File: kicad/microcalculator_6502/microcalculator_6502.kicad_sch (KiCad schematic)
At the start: 51 parts, among them J1 /SO, J10 CA, J11 IRQ_EXT_0, J12 IRQ_EXT_1, J13 CB, J14 D[7...0], J15 AUXILIARE, J16 RX_C, J17 TX_D, J18 RX_D, J2 A[11...0], J3 A[15...12], J4 D[7...0], J5 /ML, J6 /VP, J7 SYNC, J8 D[7...0], J9 /NMI, SW1 RESET, U1 65C02, U2 65C22, U3 65C51, U4 62256, U5 28C256, U6 74LS08, U7 74LS73, U8 ATF22V10C-15PU, Y1 CXO_DIP14, Y2 CXO_DIP8

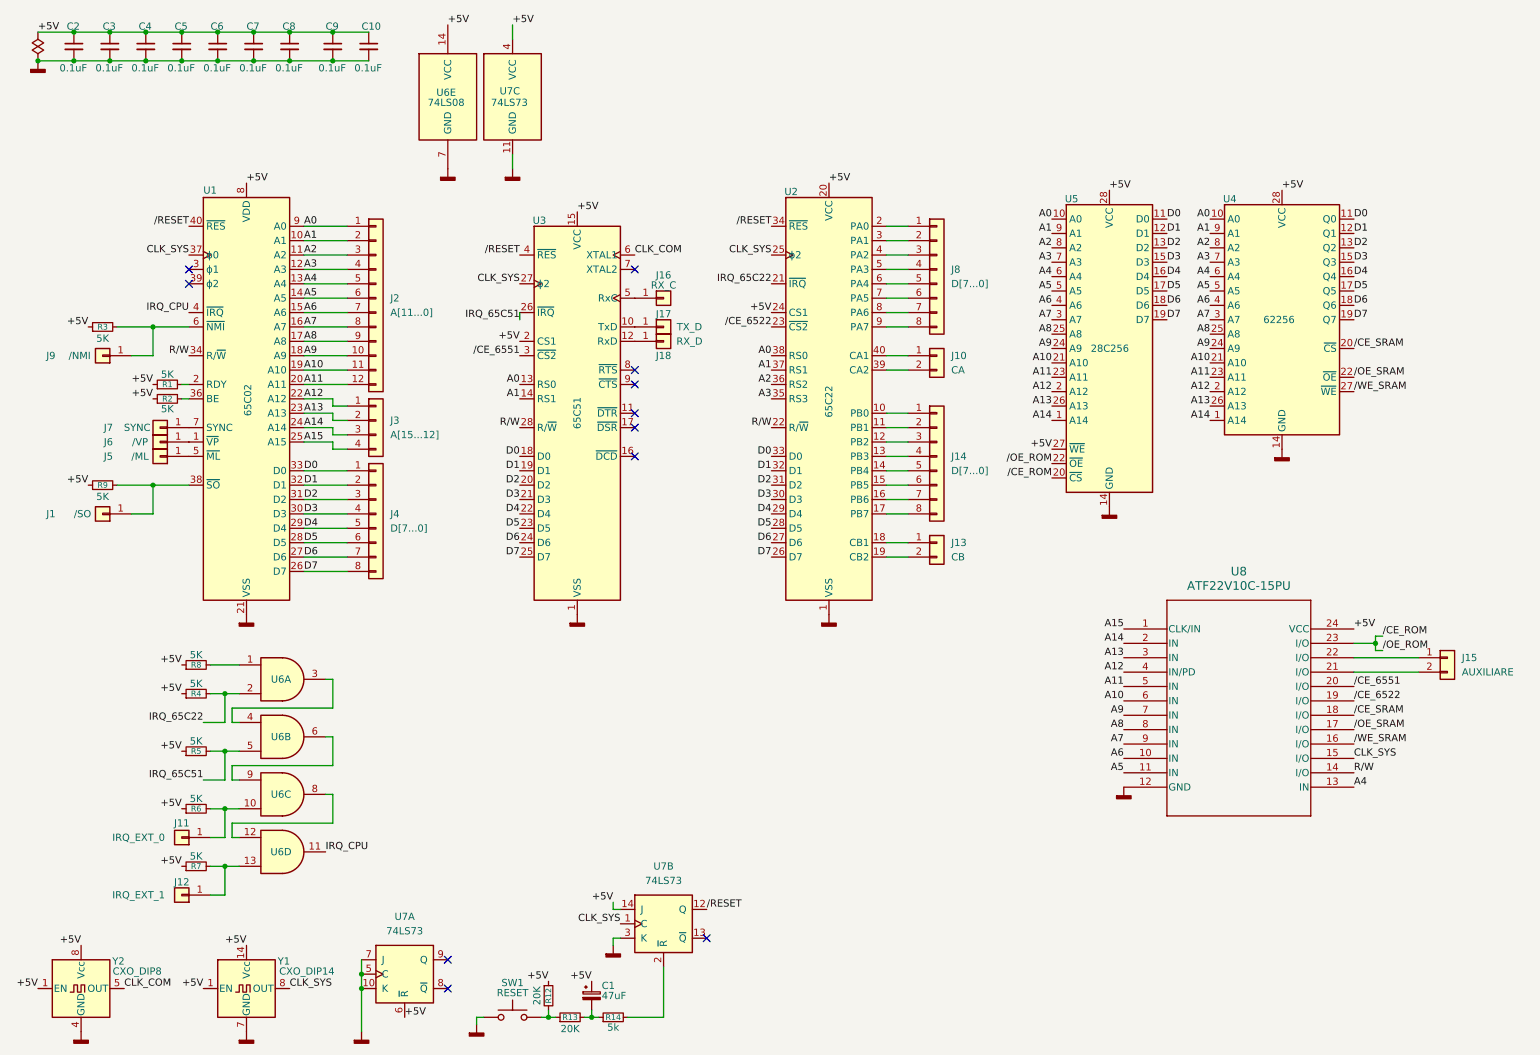
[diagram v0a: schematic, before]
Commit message: diagrama actualizata
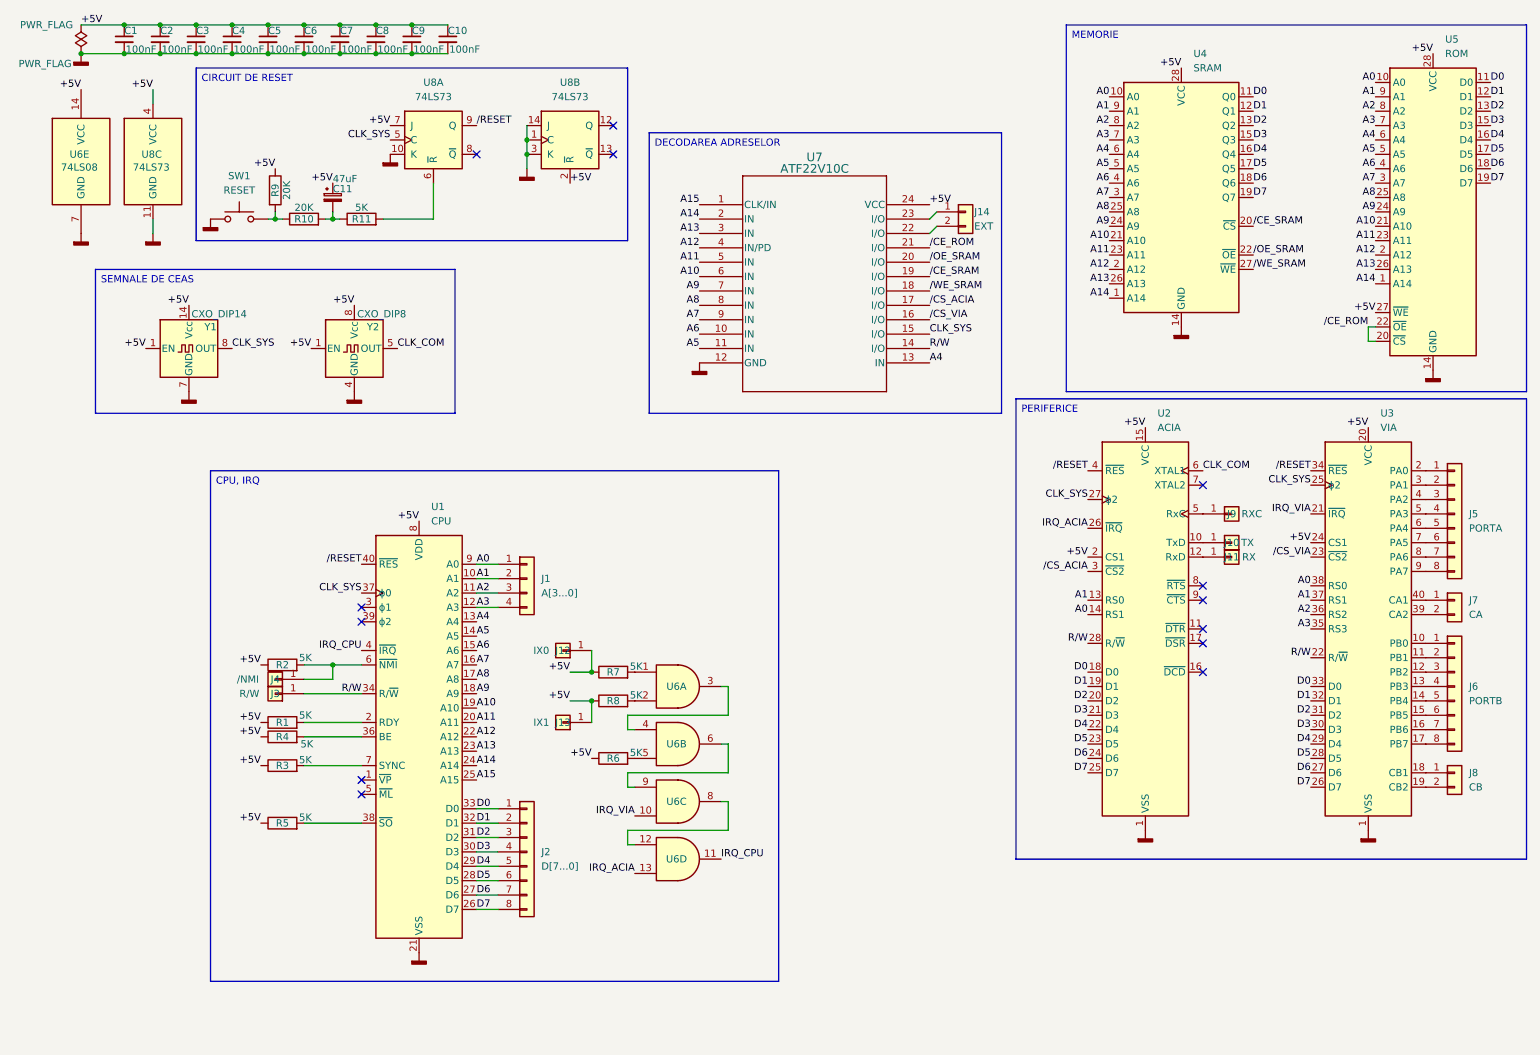
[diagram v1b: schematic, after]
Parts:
- removed C1: 47uF, symbol Device:C_Polarized_Small
- removed J1: /SO, symbol Connector_Generic:Conn_01x01
- removed J10: CA, symbol Connector_Generic:Conn_01x02
- removed J13: CB, symbol Connector_Generic:Conn_01x02
- removed J14, J4, J8: D[7...0], symbol Connector_Generic:Conn_01x08
- removed J15: AUXILIARE, symbol Connector_Generic:Conn_01x02
- removed J16: RX_C, symbol Connector_Generic:Conn_01x01
- removed J17: TX_D, symbol Connector_Generic:Conn_01x01
- removed J18: RX_D, symbol Connector_Generic:Conn_01x01
- removed J2: A[11...0], symbol Connector_Generic:Conn_01x12
- removed J3: A[15...12], symbol Connector_Generic:Conn_01x04
- removed J5: /ML, symbol Connector_Generic:Conn_01x01
- removed J6: /VP, symbol Connector_Generic:Conn_01x01
- removed J7: SYNC, symbol Connector_Generic:Conn_01x01
- removed R1, R2, R3, R4, R5, R6, R7, R8, R9: 5K, symbol Device:R_Small
- removed R12, R13: 20K, symbol Device:R_Small
- removed R14: 5k, symbol Device:R_Small
- removed U2: 65C22, Package_DIP:DIP-40_W15.24mm, symbol PCM_65xx-library:W65C22SxP
- removed U3: 65C51, Package_DIP:DIP-28_W15.24mm, symbol PCM_65xx-library:W65C51NxP
- removed U7: 74LS73, symbol 74xx:74LS73
- removed U8: ATF22V10C-15PU, 24P3_ATM, symbol ATF22V10:ATF22V10C-15PU
- added C1: 100nF, Capacitor_THT:C_Disc_D3.0mm_W2.0mm_P2.50mm, symbol Device:C_Small
- added C11: 47uF, Capacitor_THT:CP_Radial_D5.0mm_P2.50mm, symbol Device:C_Polarized_Small
- added J1: A[3...0], Connector_PinHeader_2.54mm:PinHeader_1x04_P2.54mm_Vertical, symbol Connector_Generic:Conn_01x04
- added J10: TX, Connector_PinHeader_2.54mm:PinHeader_1x01_P2.54mm_Vertical, symbol Connector_Generic:Conn_01x01
- added J13: IX1, Connector_PinHeader_2.54mm:PinHeader_1x01_P2.54mm_Vertical, symbol Connector_Generic:Conn_01x01
- added J14: EXT, Connector_PinHeader_2.54mm:PinHeader_1x02_P2.54mm_Vertical, symbol Connector_Generic:Conn_01x02
- added J2: D[7...0], Connector_PinHeader_2.54mm:PinHeader_1x08_P2.54mm_Vertical, symbol Connector_Generic:Conn_01x08
- added J3: R/W, Connector_PinHeader_2.54mm:PinHeader_1x01_P2.54mm_Vertical, symbol Connector_Generic:Conn_01x01
- added J4: /NMI, Connector_PinHeader_2.54mm:PinHeader_1x01_P2.54mm_Vertical, symbol Connector_Generic:Conn_01x01
- added J5: PORTA, Connector_PinHeader_2.54mm:PinHeader_1x08_P2.54mm_Vertical, symbol Connector_Generic:Conn_01x08
- added J6: PORTB, Connector_PinHeader_2.54mm:PinHeader_1x08_P2.54mm_Vertical, symbol Connector_Generic:Conn_01x08
- added J7: CA, Connector_PinHeader_2.54mm:PinHeader_1x02_P2.54mm_Vertical, symbol Connector_Generic:Conn_01x02
- added J8: CB, Connector_PinHeader_2.54mm:PinHeader_1x02_P2.54mm_Vertical, symbol Connector_Generic:Conn_01x02
- added R1, R11, R2, R3, R4, R5, R6, R7, R8: 5K, Resistor_THT:R_Axial_DIN0207_L6.3mm_D2.5mm_P2.54mm_Vertical, symbol Device:R
- added R10, R9: 20K, Resistor_THT:R_Axial_DIN0207_L6.3mm_D2.5mm_P2.54mm_Vertical, symbol Device:R
- added U2: ACIA, Package_DIP:DIP-28_W15.24mm, symbol PCM_65xx-library:W65C51NxP
- added U3: VIA, Package_DIP:DIP-40_W15.24mm, symbol PCM_65xx-library:W65C22NxP
- added U7: ATF22V10C, Package_DIP:DIP-24_W7.62mm, symbol ATF:ATF22V10C-15PU
- added U8: 74LS73, Package_DIP:DIP-14_W7.62mm, symbol 74xx:74LS73
- C10, C2, C3, C4, C5, C6, C7, C8, C9: value 0.1uF -> 100nF; footprint (none) -> Capacitor_THT:C_Disc_D3.0mm_W2.0mm_P2.50mm
- J11: value IRQ_EXT_0 -> RX; footprint (none) -> Connector_PinHeader_2.54mm:PinHeader_1x01_P2.54mm_Vertical
- J12: value IRQ_EXT_1 -> IX0; footprint (none) -> Connector_PinHeader_2.54mm:PinHeader_1x01_P2.54mm_Vertical
- J9: value /NMI -> RXC; footprint (none) -> Connector_PinHeader_2.54mm:PinHeader_1x01_P2.54mm_Vertical
- SW1: footprint (none) -> Button_Switch_THT:SW_PUSH_6mm
- U1: value 65C02 -> CPU
- U4: value 62256 -> SRAM
- U5: value 28C256 -> ROM; footprint (none) -> Package_DIP:DIP-28_W15.24mm
- U6: footprint (none) -> Package_DIP:DIP-14_W7.62mm
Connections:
- net +5V: now also J12.1 (Pin_1), C1.1, C11.1, J13.1 (Pin_1), R1.1, R2.1, R3.1, R4.1, R5.1, R6.1, R7.1, R8.1, R9.1, U2.15 (VCC), U2.2 (CS1), U3.20 (VCC), U3.24 (CS1), U7.24 (VCC), U8.2 (~{R}), U8.4 (VCC), U8.7 (J)
- net A0: now also J1.1 (Pin_1), U2.14 (RS1), U3.38 (RS0)
- net A1: now also J1.2 (Pin_2), U2.13 (RS0), U3.37 (RS1)
- net A10: now also U7.6 (IN)
- net A11: now also U7.5 (IN)
- net A12: now also U7.4 (IN/PD)
- net A13: now also U7.3 (IN)
- net A14: now also U7.2 (IN)
- net A15: now also U7.1 (CLK/IN)
- net A2: now also J1.3 (Pin_3), U3.36 (RS2)
- net A3: now also J1.4 (Pin_4), U3.35 (RS3)
- net A4: now also U7.13 (IN)
- net A5: now also U7.11 (IN)
- net A6: now also U7.10 (IN)
- net A7: now also U7.9 (IN)
- net A8: now also U7.8 (IN)
- net A9: now also U7.7 (IN)
- net CLK_COM: now also U2.6 (XTAL1)
- net CLK_SYS: now also U2.27 (ϕ2), U3.25 (ϕ2), U7.15 (I/O), U8.5 (C)
- net D0: now also J2.1 (Pin_1), U2.18 (D0), U3.33 (D0)
- net D1: now also J2.2 (Pin_2), U2.19 (D1), U3.32 (D1)
- net D2: now also J2.3 (Pin_3), U2.20 (D2), U3.31 (D2)
- net D3: now also J2.4 (Pin_4), U2.21 (D3), U3.30 (D3)
- net D4: now also J2.5 (Pin_5), U2.22 (D4), U3.29 (D4)
- net D5: now also J2.6 (Pin_6), U2.23 (D5), U3.28 (D5)
- net D6: now also J2.7 (Pin_7), U2.24 (D6), U3.27 (D6)
- net D7: now also J2.8 (Pin_8), U2.25 (D7), U3.26 (D7)
- net GNDD: now also C1.2, U2.1 (VSS), U3.1 (VSS), U7.12 (GND), U8.1 (C), U8.10 (K), U8.11 (GND), U8.14 (J), U8.3 (K)
- net R/W: now also J3.1 (Pin_1), U2.28 (R/~{W}), U3.22 (R/~{W}), U7.14 (I/O)
- net /CE_ROM: now also U7.21 (I/O)
- net /CE_SRAM: now also U7.19 (I/O)
- net /OE_SRAM: now also U7.20 (I/O)
- net /RESET: now also U2.4 (~{RES}), U3.34 (~{RES}), U8.9 (Q)
- net /WE_SRAM: now also U7.18 (I/O)
- net at SW1.2: now also R10.1, R9.2
- net at U1.2 (RDY): now also R1.2
- net at U1.36 (BE): now also R4.2
- net at U1.38 (~{SO}): now also R5.2
- net at U1.6 (~{NMI}): now also J4.1 (Pin_1), R2.2; no longer J9.1 (Pin_1)
- net at U1.7 (SYNC): now also R3.2
- net at J11.1 (Pin_1): now also U2.12 (RxD); no longer U6.10
- net IRQ_ACIA: now reaches U6.13
- net IRQ_ACIA: now also U2.26 (~{IRQ}); no longer J12.1 (Pin_1)
- net at U6.1: now also R7.2
- net IRQ_65C22: no longer names the net of U6.2
- net IRQ_65C22: now also R8.2
- net IRQ_65C51: no longer names the net of U6.5
- net IRQ_65C51: now also R6.2
- new net: J6.1 (Pin_1), U3.10 (PB0)
- new net: J6.2 (Pin_2), U3.11 (PB1)
- new net: J6.3 (Pin_3), U3.12 (PB2)
- new net: J6.4 (Pin_4), U3.13 (PB3)
- new net: J6.5 (Pin_5), U3.14 (PB4)
- new net: J6.6 (Pin_6), U3.15 (PB5)
- new net: J6.7 (Pin_7), U3.16 (PB6)
- new net: J6.8 (Pin_8), U3.17 (PB7)
- new net: J8.1 (Pin_1), U3.18 (CB1)
- new net: J8.2 (Pin_2), U3.19 (CB2)
- new net: J5.1 (Pin_1), U3.2 (PA0)
- new net: J5.2 (Pin_2), U3.3 (PA1)
- new net: J7.2 (Pin_2), U3.39 (CA2)
- new net: J5.3 (Pin_3), U3.4 (PA2)
- new net: J7.1 (Pin_1), U3.40 (CA1)
- new net: J5.4 (Pin_4), U3.5 (PA3)
- new net: J5.5 (Pin_5), U3.6 (PA4)
- new net: J5.6 (Pin_6), U3.7 (PA5)
- new net: J5.7 (Pin_7), U3.8 (PA6)
- new net: J5.8 (Pin_8), U3.9 (PA7)
- new net: R11.2, U8.6 (~{R})
- new net: C11.2, R10.2, R11.1
- new net: J10.1 (Pin_1), U2.10 (TxD)
- new net: J14.1 (Pin_1), U7.23 (I/O)
- new net: J14.2 (Pin_2), U7.22 (I/O)
- new net: J9.1 (Pin_1), U2.5 (RxC)
- new net IRQ_VIA: U3.21 (~{IRQ}), U6.10
- new net /CS_ACIA: U2.3 (~{CS2}), U7.17 (I/O)
- new net /CS_VIA: U3.23 (~{CS2}), U7.16 (I/O)
- no-connect marks 11 -> 13
